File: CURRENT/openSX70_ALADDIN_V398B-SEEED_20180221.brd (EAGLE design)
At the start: 95.9 x 27.9 mm, 45 parts, among them Q1 5.8A/30V/35mΩ, Q2 5.8A/30V/35mΩ, U1 ATMEGA328P_TQFP, U3 BH1750FVI-TR, Y1 CSTCE8M00G52Z-R0

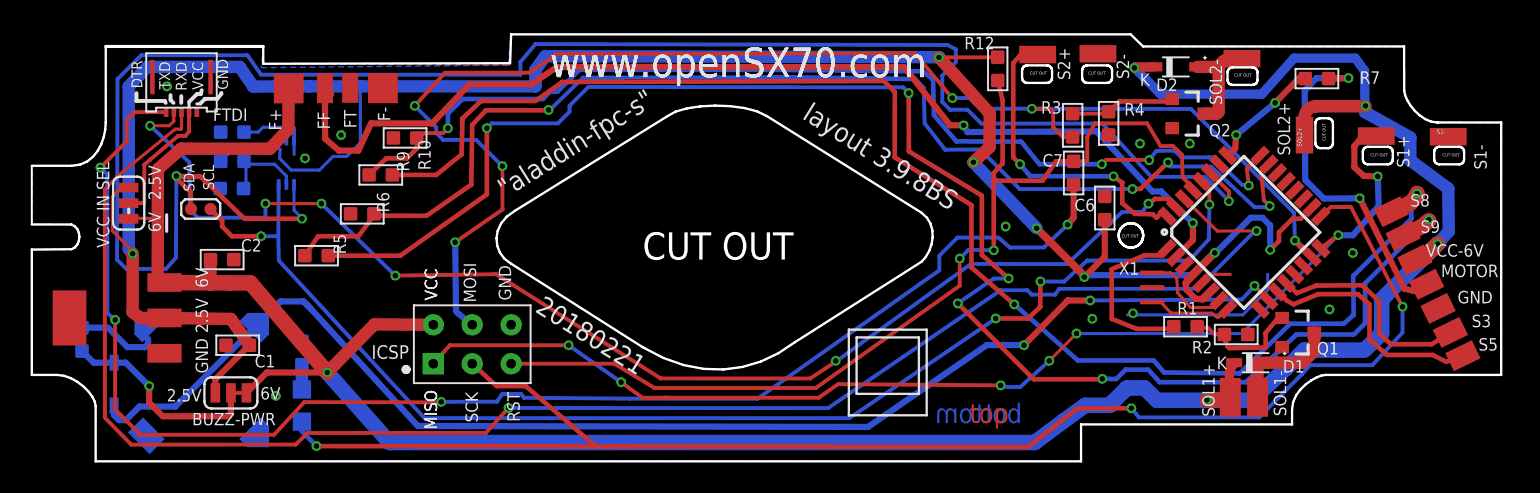
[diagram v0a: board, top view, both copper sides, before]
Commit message: And so on...
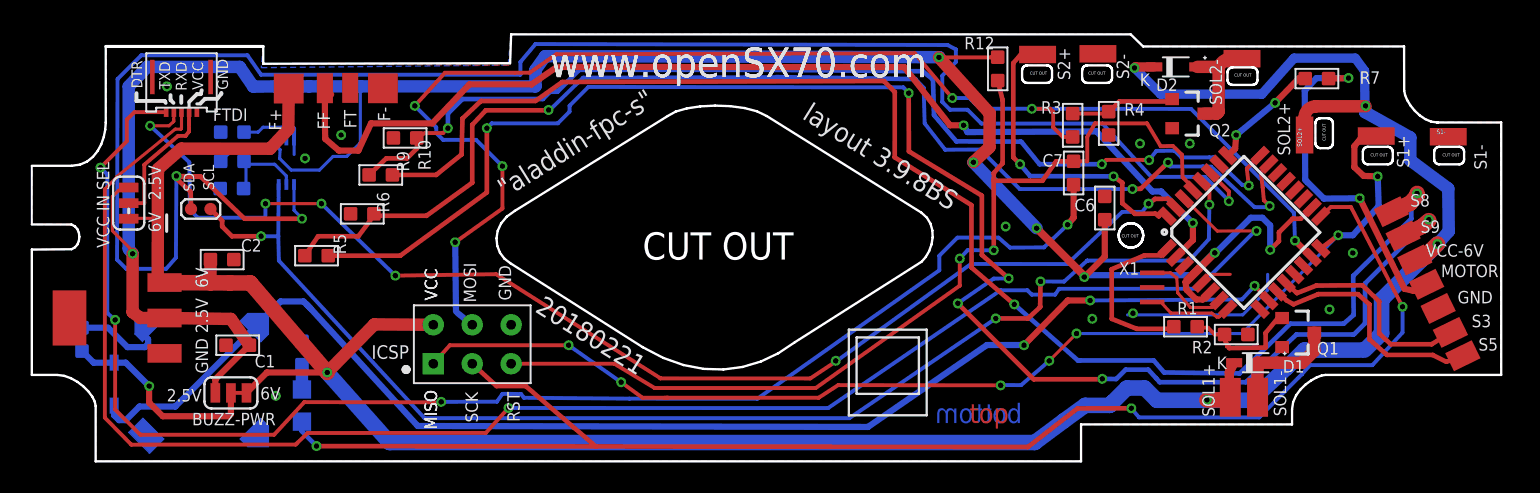
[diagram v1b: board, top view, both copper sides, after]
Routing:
- net 6V: track 209.4 -> 205.4 mm
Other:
- board text added: "B-"
